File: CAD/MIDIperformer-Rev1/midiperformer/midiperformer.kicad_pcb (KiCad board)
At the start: 2 copper layers, 89.8 x 65 mm, 41 parts, among them J1 MIDI IN B, J2 MIDI IN A, J3 MIDI OUT A, J4 MIDI OUT B, J5 Barrel_Jack, SW1 SW_Push_SPDT, SW3 SW_Push_SPDT, SW4 SW_Push_SPDT, SW5 SW_Push_SPDT, SW6 SW_Push_SPDT, SW7 SW_Push_SPDT, SW8 SW_Push_SPDT, U1 6N138, U2 6N138, U3 L7805, U4 Teensy-LC, U5 WS2812, U6 MCP23017_SP

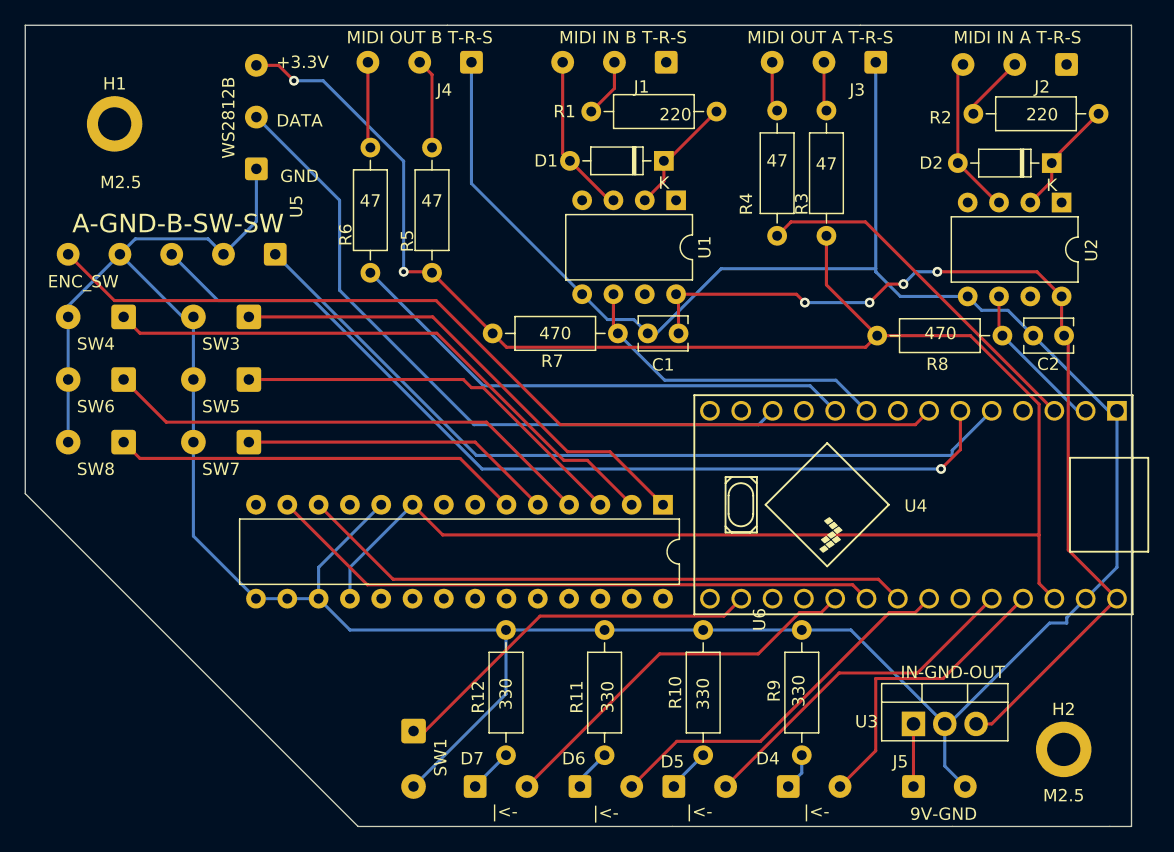
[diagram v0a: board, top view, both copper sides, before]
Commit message: progress on midiperformer; this one is being printed progress on clarinoid3 schematic; very WIP
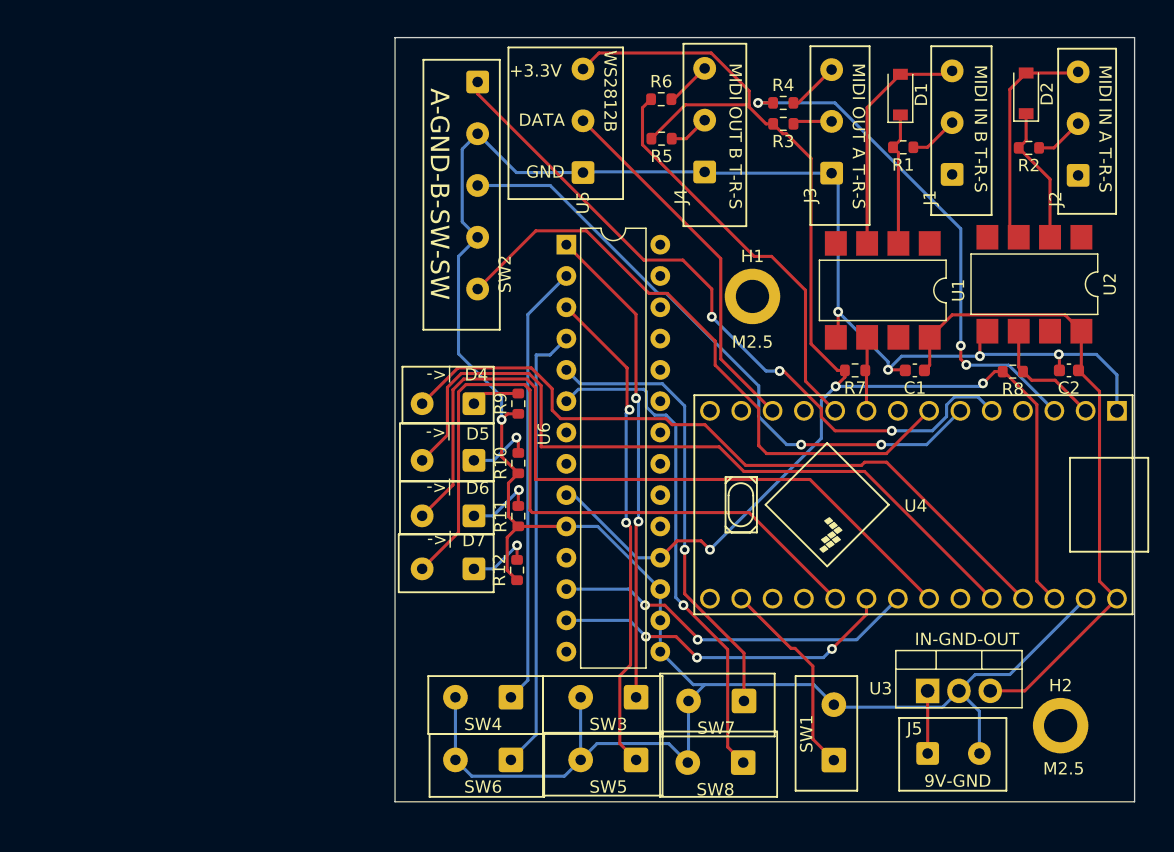
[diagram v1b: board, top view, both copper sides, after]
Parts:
- C1, C2: footprint Capacitor_THT:C_Disc_D3.8mm_W2.6mm_P2.50mm -> Capacitor_SMD:C_0603_1608Metric
- D1, D2: footprint Diode_THT:D_DO-35_SOD27_P7.62mm_Horizontal -> Diode_SMD:D_SOD-123
- R1, R10, R11, R12, R2, R3, R4, R5, R6, R7, R8, R9: footprint Resistor_THT:R_Axial_DIN0207_L6.3mm_D2.5mm_P10.16mm_Horizontal -> Resistor_SMD:R_0603_1608Metric
- U1, U2: footprint Package_DIP:DIP-8_W7.62mm -> Package_DIP:SMDIP-8_W7.62mm
- moved SW8 56.6 mm to (212.2, 109.8)
- moved H1 53.6 mm to (213.0, 72.0)
- moved SW7 45.3 mm to (212.3, 104.8)
- moved SW3 44.0 mm to (203.6, 104.5)
- moved SW4 44.0 mm to (193.4, 104.5)
- moved SW5 44.0 mm to (203.6, 109.6)
- moved SW6 44.0 mm to (193.4, 109.6)
- moved D4 40.2 mm to (190.4, 80.7), turned to 180 degrees
- moved SW1 34.2 mm to (219.6, 109.6), turned to 90 degrees
- moved D5 31.0 mm to (190.4, 85.3), turned to 180 degrees
- moved R9 29.4 mm to (194.0, 80.7), turned to 90 degrees
- moved R6 27.5 mm to (205.6, 56.0), turned to 0 degrees
- moved U5 26.5 mm to (199.2, 62.0)
- moved R1 25.5 mm to (225.2, 59.9), turned to 180 degrees
- moved J1 24.9 mm to (229.2, 62.1), turned to 90 degrees
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- renumbered ENC_SW to SW2
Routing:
- net GND: track 282.9 -> 223.4 mm, vias 0 -> 5
- net +3V3: track 168.6 -> 119.1 mm, vias 2 -> 3
- net Net-(D4-Pad2): track 24.6 -> 58.9 mm
- net Net-(D5-Pad2): track 27.9 -> 61.9 mm
- net Net-(D6-Pad2): track 30.4 -> 62.0 mm
- net Net-(D7-Pad2): track 31.3 -> 59.3 mm
- net Net-(U4-Pad12): track 57.0 -> 29.9 mm
- net +5V: track 78.7 -> 52.9 mm, vias 4 -> 0
- net Net-(SW2-Pad5): track 76.0 -> 50.4 mm
- net Net-(SW2-Pad3): track 75.0 -> 50.5 mm, vias 1 -> 2
- net Net-(U4-Pad25): track 50.1 -> 28.3 mm, vias 0 -> 3
- net Net-(U4-Pad26): track 50.1 -> 30.0 mm, vias 0 -> 2
- net Net-(R7-Pad1): track 26.1 -> 6.06 mm
- net Net-(SW1-Pad1): track 31.0 -> 16.4 mm
- net Net-(R4-Pad1): track 29.3 -> 41.8 mm, vias 0 -> 3
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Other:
- board size 89.8 x 65 mm -> 60 x 62 mm
- board text removed: "220"
- board text removed: "330"
- board text removed: "47"
- board text removed: "470"
